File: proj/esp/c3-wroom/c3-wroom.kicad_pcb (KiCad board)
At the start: 2 copper layers, 20.3 x 34.3 mm, 13 parts, among them J1 USB-C, J2 Conn_01x08_Pin, J3 Conn_01x01_Pin, J4 Conn_01x08_Pin, U1 ESP32-C3-WROOM-02, U2 LM1117MP-3.3, U3 WS2812C

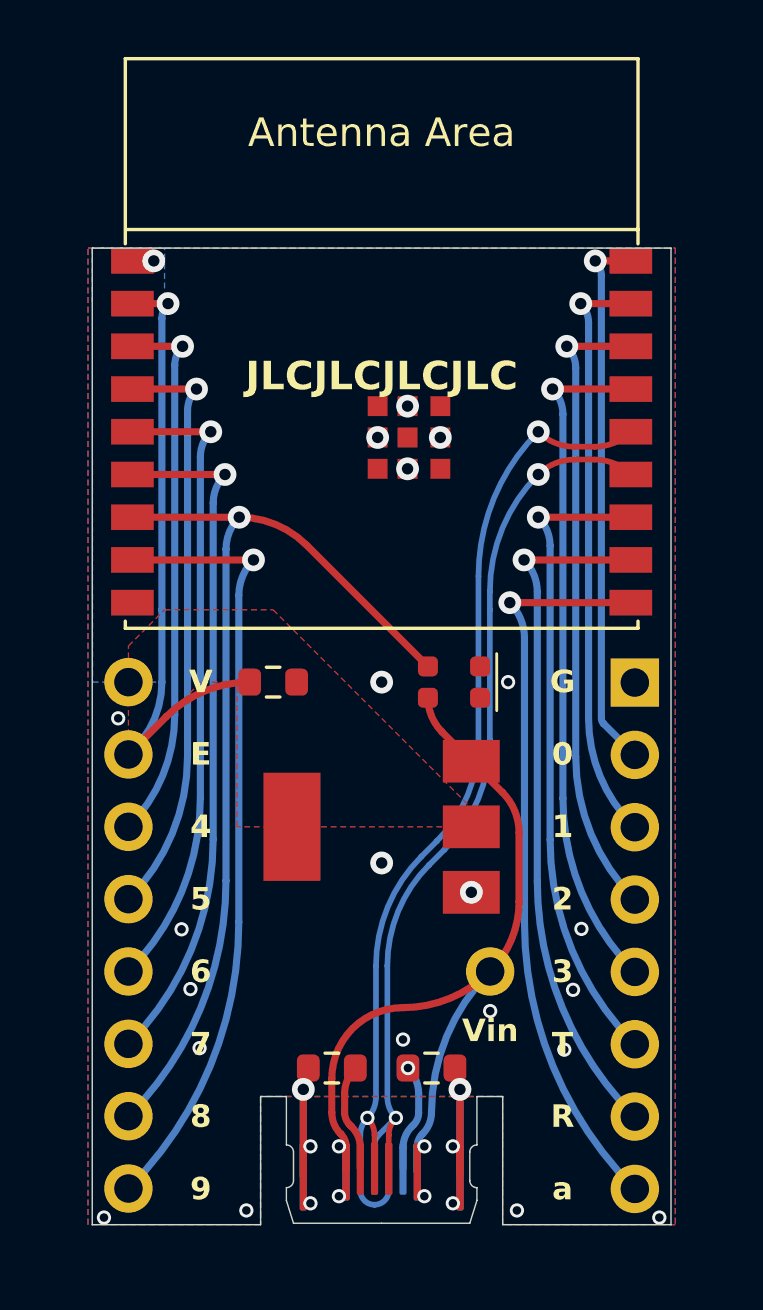
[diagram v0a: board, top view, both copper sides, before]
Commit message: -
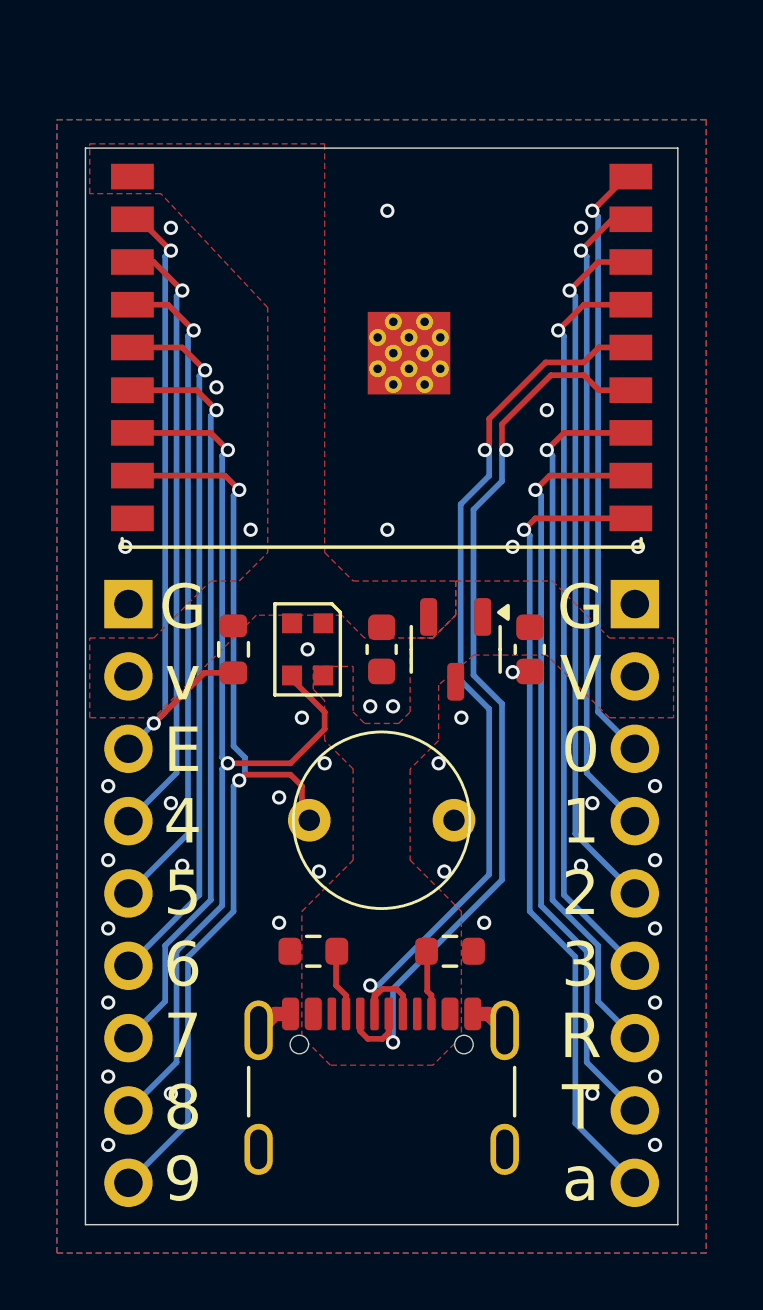
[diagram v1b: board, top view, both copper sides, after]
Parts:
- removed the ? at (100.0, 89.8)
- removed the G*** at (97.5, 68.2)
- removed the G*** at (102.5, 68.2)
- removed J4: Conn_01x08_Pin, Connector_PinHeader_2.54mm:PinHeader_1x08_P2.54mm_Vertical
- removed U3: WS2812C, Library:WS2812C-2020
- added ?: , Library:PCB.MCBEERINGI.DEV_small, B.Cu at (98.8, 77.8)
- added C1: 1u, Capacitor_SMD:C_0603_1608Metric, F.Cu at (105.2, 79.8)
- added C2: 1u, Capacitor_SMD:C_0603_1608Metric, F.Cu at (100.0, 79.8)
- added D1: WS2812B-2020, LED_SMD:LED_WS2812B-2020_PLCC4_2.0x2.0mm, F.Cu at (97.4, 79.8)
- added G***: LOGO, LOGO, B.Cu at (100.0, 68.8)
- added SW1: SW_BOOT, Library:alps-skrg, F.Cu at (100.0, 85.8)
- J1: value USB-C -> USB_C_Receptacle_USB2.0_16P; footprint Library:USB-C -> Connector_USB:USB_C_Receptacle_GCT_USB4105-xx-A_16P_TopMnt_Horizontal
- J2: value Conn_01x08_Pin -> OUT1; footprint Connector_PinHeader_2.54mm:PinHeader_1x08_P2.54mm_Vertical -> Connector_PinHeader_2.54mm:PinHeader_1x09_P2.54mm_Vertical
- J3: value Conn_01x01_Pin -> OUT2; footprint Connector_PinHeader_2.54mm:PinHeader_1x01_P2.54mm_Vertical -> Connector_PinHeader_2.54mm:PinHeader_1x09_P2.54mm_Vertical
- U1: footprint PCM_Espressif:ESP32-C3-WROOM-02 -> RF_Module:ESP32-C3-WROOM-02
- U2: value LM1117MP-3.3 -> AP7333; footprint Package_TO_SOT_SMD:SOT-223-3_TabPin2 -> Package_TO_SOT_SMD:SOT-23-3
- moved J3 13.9 mm to (108.9, 78.2)
- moved U2 6.75 mm to (102.6, 79.8), turned to -90 degrees
- moved R2 5.83 mm to (97.6, 90.4), turned to 180 degrees
- moved R3 5.83 mm to (102.4, 90.4), turned to 0 degrees
- moved U1 2.86 mm to (100.0, 69.2)
- moved J2 2.74 mm to (91.1, 78.2)
- moved R1 1.80 mm to (94.8, 79.8), turned to -90 degrees
- moved J1 0.78 mm to (100.0, 96.3), turned to 0 degrees
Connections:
- J2 pad 1: +3.3V -> GND
- J2 pad 2: EN -> +3.3V
- J2 pad 3: IO4 -> EN
- J2 pad 4: IO5 -> IO4
- J2 pad 5: IO6 -> IO5
- J2 pad 6: IO7 -> IO6
- J2 pad 7: IO8 -> IO7
- J2 pad 8: IO9 -> IO8
- J3 pad 1: +5V -> GND
- R2 pad 1: Net-(J1-CC2) -> Net-(J1-CC1)
- R3 pad 1: Net-(J1-CC1) -> Net-(J1-CC2)
- U2 pad 1: GND -> VBUS
- U2 pad 3: +5V -> GND
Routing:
- net +5V: track 29.3 -> 0.00 mm, vias 4 -> 0
- net GND: track 12.2 -> 2.72 mm, vias 27 -> 41
- net IO9: track 27.4 -> 34.0 mm, vias 1 -> 2
- net D+: track 36.0 -> 32.3 mm
- net TXD: track 22.6 -> 25.1 mm
- net RXD: track 24.3 -> 26.8 mm
- net IO10: track 25.9 -> 28.5 mm
- net IO5: track 20.8 -> 23.2 mm
- net IO6: track 22.4 -> 24.9 mm
- net IO7: track 24.1 -> 26.6 mm
- net IO2: track 22.3 -> 24.7 mm
- net IO3: track 23.9 -> 26.3 mm
- net IO4: track 19.2 -> 21.6 mm
- net IO0: track 19.1 -> 21.4 mm
- net IO1: track 21.0 -> 23.0 mm
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- added copper zone on F.Cu, net VBUS
- removed copper zone on B.Cu, net +3.3V
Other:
- board size 20.3 x 34.3 mm -> 20.8 x 37.8 mm
- board text added: "ESP32 C3 dev board"
- board text added: "ESP32-C3 WROOM-02"
- board text added: "G V 0 1 2 3 R T a"
- board text added: "G v E 4 5 6 7 8 9"
- board text removed: "G 0 1 2 3 T R a"
- board text removed: "JLCJLCJLCJLC"
- board text removed: "V E 4 5 6 7 8 9"
- board text removed: "Vin"

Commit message: -
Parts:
- J2, J3: moved to B.Cu
- turned J2 to 180 degrees
- turned J3 to 180 degrees
